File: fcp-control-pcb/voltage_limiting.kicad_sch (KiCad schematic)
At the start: 15 parts, among them J8 LimiterBypass, Q1 AONR21321, U2 LM311DR

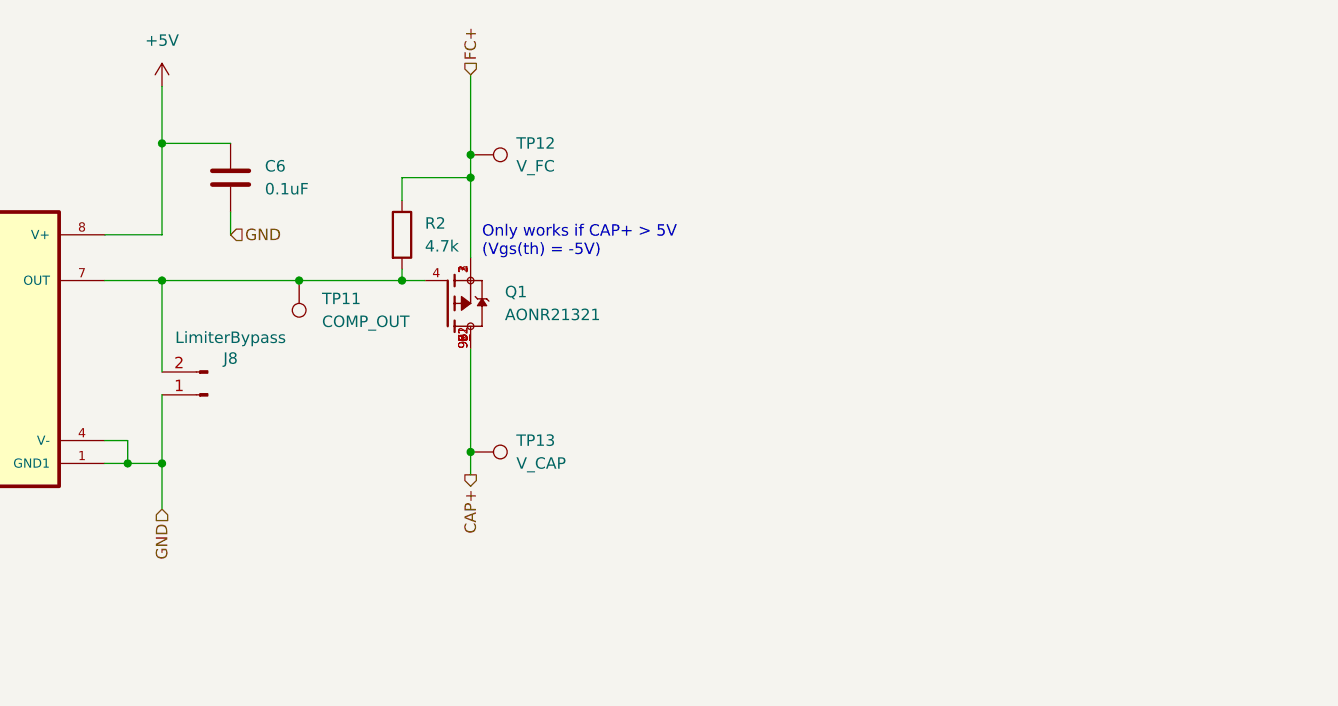
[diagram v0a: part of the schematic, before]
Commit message: queen r1.1
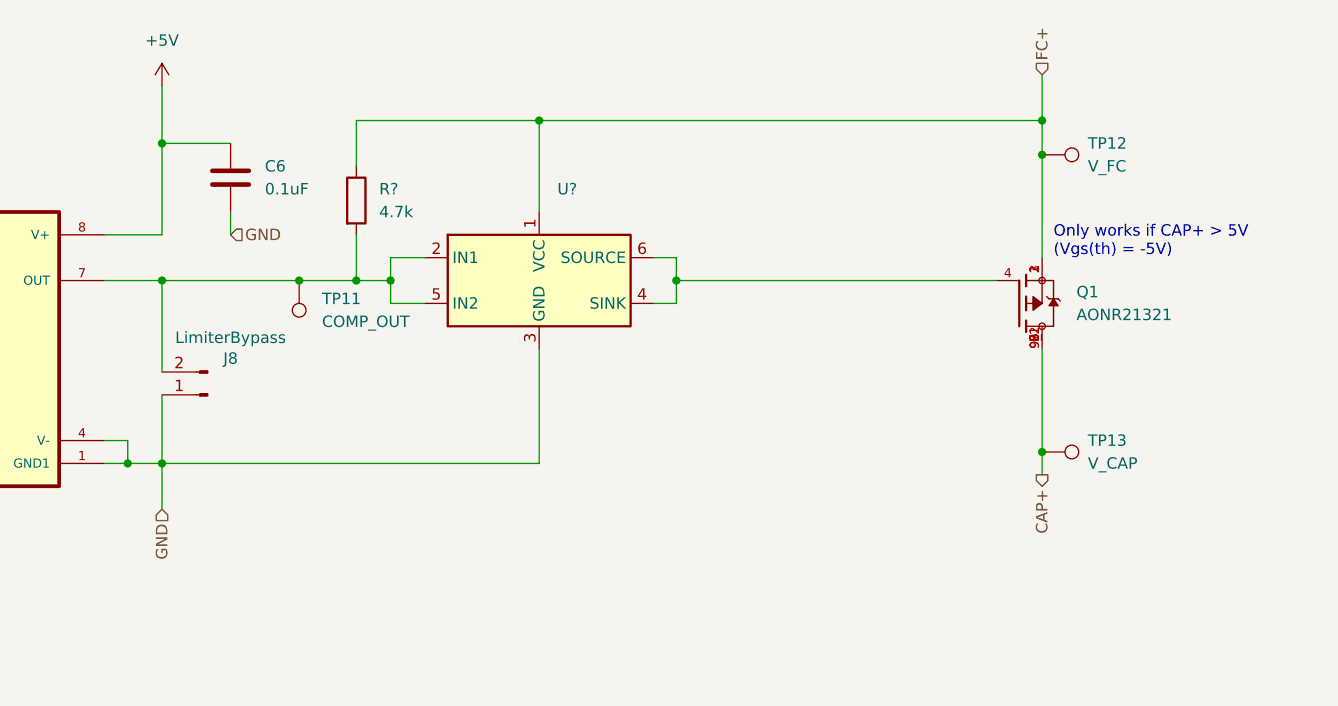
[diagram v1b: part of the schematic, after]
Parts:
- removed R2: 4.7k, Resistor_SMD:R_0805_2012Metric_Pad1.20x1.40mm_HandSolder, symbol Device:R
- added R?: 4.7k, Resistor_SMD:R_0805_2012Metric_Pad1.20x1.40mm_HandSolder, symbol Device:R
- added U?: (no value), symbol Driver_FET:ZXGD3003E6
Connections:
- net CHRG-: now also U?.3 (GND)
- net FC+: now also R?.1, U?.1 (VCC)
- net at J8.2 (Pin_2), TP11.1, U2.7 (OUT): now also R?.2, U?.2 (IN1), U?.5 (IN2); no longer Q1.4
- new net: Q1.4, U?.4 (SINK), U?.6 (SOURCE)
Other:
- moved on the sheet: Q1, TP12, TP13
